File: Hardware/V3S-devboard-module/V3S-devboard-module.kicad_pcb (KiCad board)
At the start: 4 copper layers, 32 x 55 mm, 86 parts, among them J101 Conn_01x02, J201 Micro_SD_Card_Det1, J301 AS0BC21-S30BE-7H, SW201 SW_MEC_5E, U101 EA3036C, U102 XC6206PxxxMR, U201 V3S, U202 W25Q128JVS, Y201 Crystal_Small, Y202 Crystal_GND24_Small

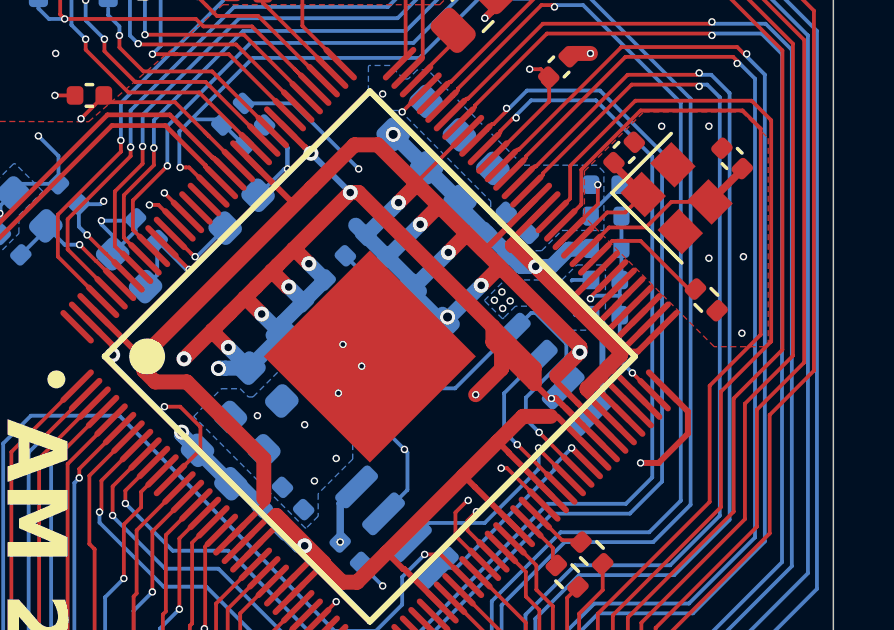
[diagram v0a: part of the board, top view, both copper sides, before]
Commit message: Minor changes. Sent to fab
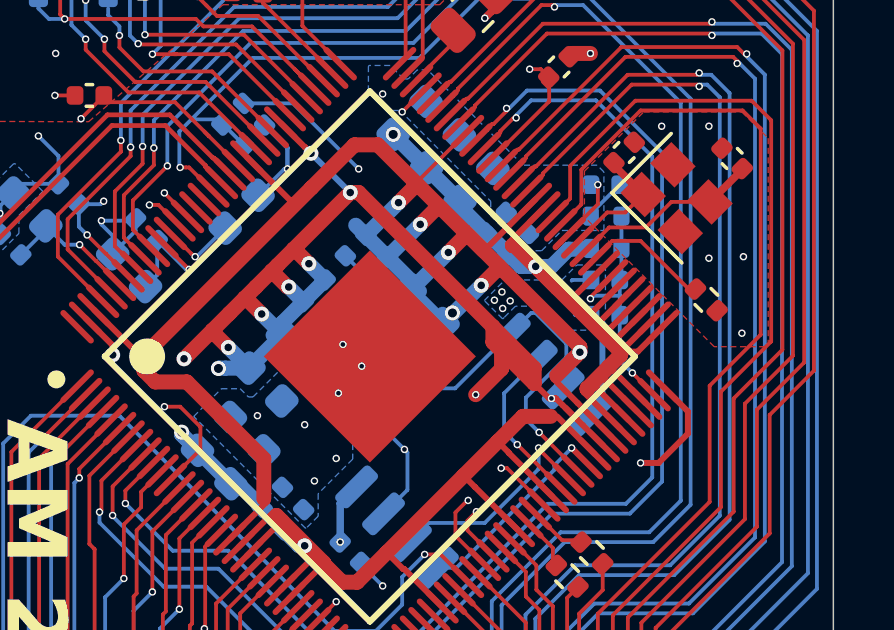
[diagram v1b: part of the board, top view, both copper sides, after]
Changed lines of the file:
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@@
 	)
 	(via
-		(at 19.138119 36.036881)
+		(at 19.3 35.9)
 		(size 0.5)
 		(drill 0.3)
@@
 		(start 10.275 39.875)
 		(end 8.925 39.875)
+		(width 0.5)
+		(layer "In1.Cu")
+		(net 2)
+	)
+	(segment
+		(start 13.325 41.85)
+		(end 9.475 41.85)
+		(width 0.5)
+		(layer "In1.Cu")
+		(net 2)
+	)
+	(segment
+		(start 19.275 35.9)
+		(end 13.325 41.85)
 		(width 0.5)
 		(layer "In1.Cu")
@@
 	)
 	(segment
-		(start 8.125 40.5)
-		(end 9.475 41.85)
+		(start 9.475 41.85)
+		(end 8.125 40.5)
 		(width 0.5)
 		(layer "In1.Cu")
@@
 	)
 	(segment
-		(start 7.575 40.5)
-		(end 2.9 35.825)
+		(start 19.3 35.9)
+		(end 19.275 35.9)
 		(width 0.5)
 		(layer "In1.Cu")
@@
 	)
 	(segment
-		(start 13.325 41.85)
-		(end 19.138119 36.036881)
+		(start 7.575 40.5)
+		(end 2.9 35.825)
 		(width 0.5)
 		(layer "In1.Cu")
@@
 		(width 0.5)
 		(layer "In1.Cu")
-		(net 2)
-	)
-	(segment
-		(start 9.475 41.85)
-		(end 13.325 41.85)
-		(width 0.5)
-		(layer "In1.Cu")
